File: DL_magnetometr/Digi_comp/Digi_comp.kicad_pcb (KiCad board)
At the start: 2 copper layers, 24 parts, among them J1 Conn_01x06_Male, U1 JST-PHR-2-Connector, U2 HC-06, U3 AP7331-WG-7, U4 ATmega328P-MU

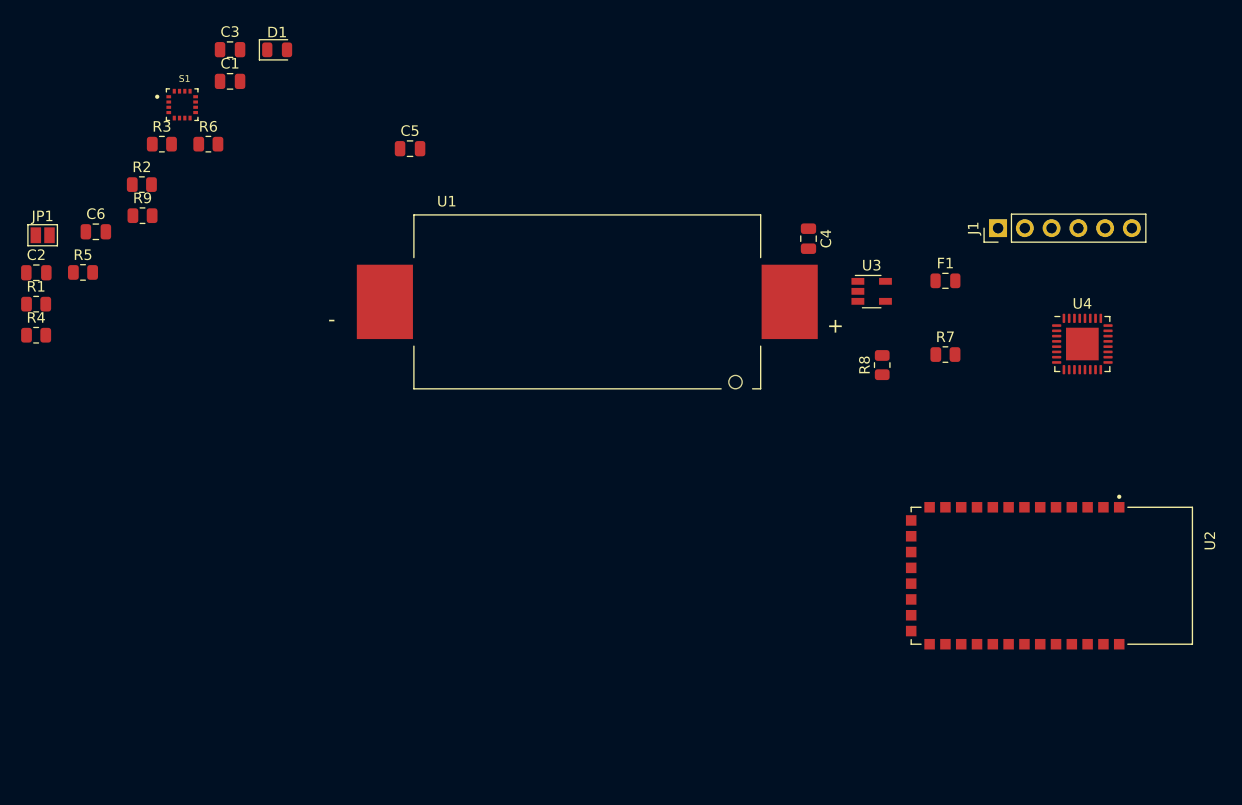
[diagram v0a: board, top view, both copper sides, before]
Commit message: Layout finished
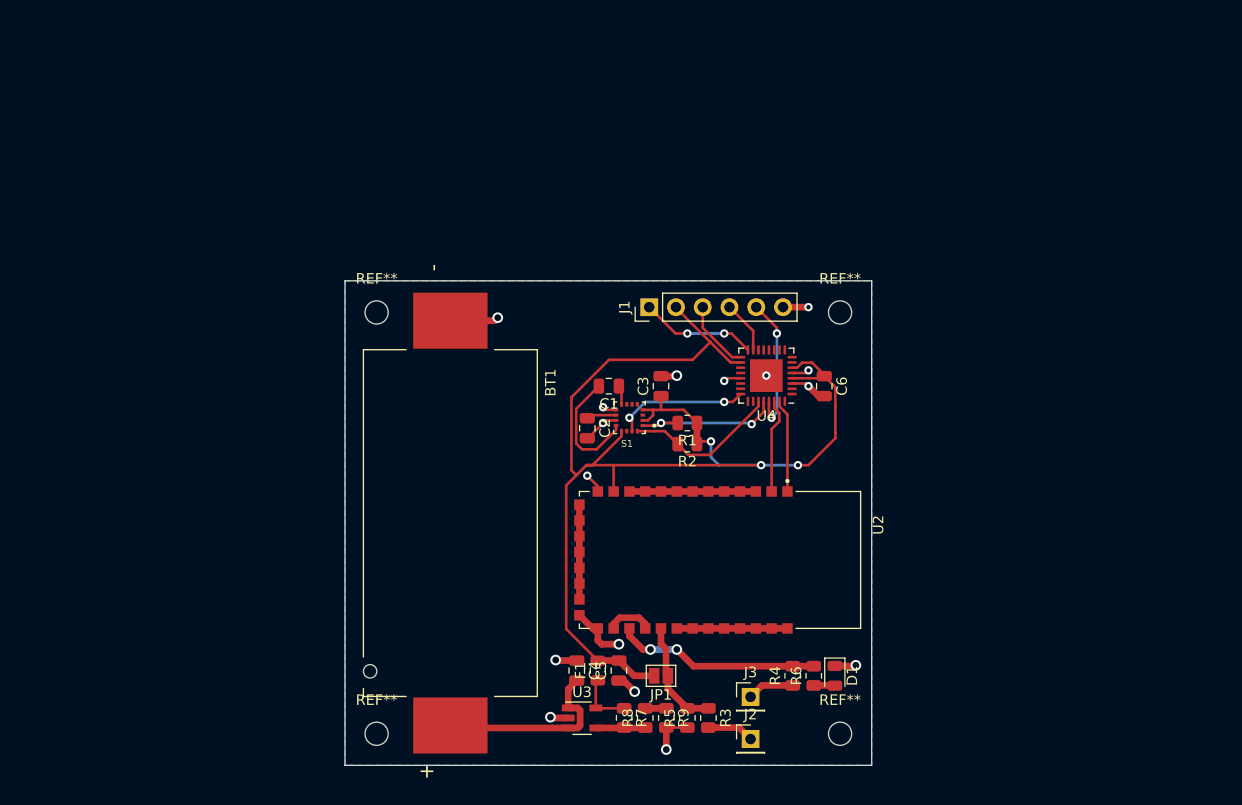
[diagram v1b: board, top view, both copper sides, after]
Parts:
- removed U1: JST-PHR-2-Connector, Dokumenty:2AA-SM
- added BT1: Battery_Cell, Dokumenty:2AA-SM, F.Cu at (75.0, 65.0)
- added J2: Conn_01x01_Male, Connector_PinHeader_2.54mm:PinHeader_1x01_P2.54mm_Vertical, F.Cu at (103.5, 85.5)
- added J3: Conn_01x01_Male, Connector_PinHeader_2.54mm:PinHeader_1x01_P2.54mm_Vertical, F.Cu at (103.5, 81.5)
- added REF**: MountingHole_2.2mm_M2, MountingHole:MountingHole_2.2mm_M2, F.Cu at (112.0, 85.0)
- added REF**: MountingHole_2.2mm_M2, MountingHole:MountingHole_2.2mm_M2, F.Cu at (68.0, 85.0)
- added REF**: MountingHole_2.2mm_M2, MountingHole:MountingHole_2.2mm_M2, F.Cu at (112.0, 45.0)
- added REF**: MountingHole_2.2mm_M2, MountingHole:MountingHole_2.2mm_M2, F.Cu at (68.0, 45.0)
- moved D1 79.6 mm to (111.5, 79.5), turned to 270 degrees
- moved R4 78.8 mm to (107.5, 79.5), turned to 90 degrees
- moved R6 76.5 mm to (109.5, 79.5), turned to 90 degrees
- moved R3 75.2 mm to (99.5, 83.5), turned to 270 degrees
- moved JP1 72.1 mm to (95.0, 79.5), turned to 180 degrees
- moved R5 71.3 mm to (97.5, 83.5), turned to 90 degrees
- moved C6 70.7 mm to (110.5, 52.0), turned to 270 degrees
- moved R9 68.9 mm to (95.5, 83.5), turned to 270 degrees
- moved R1 62.8 mm to (97.5, 55.5), turned to 180 degrees
- moved R2 57.3 mm to (97.5, 57.5), turned to 180 degrees
- moved C2 54.3 mm to (88.0, 56.0), turned to 270 degrees
- moved C5 53.4 mm to (91.0, 79.0), turned to 90 degrees
- moved C3 51.9 mm to (95.0, 52.0), turned to 90 degrees
- moved S1 51.8 mm to (92.0, 55.0), turned to 180 degrees
- moved F1 49.6 mm to (89.0, 79.0), turned to 90 degrees
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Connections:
- R3 pad 2: (no net) -> Net-(J2-Pad1)
- R4 pad 1: (no net) -> Net-(J3-Pad1)
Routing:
- net 3.3V: track 0.00 -> 122.0 mm, vias 0 -> 3
- net GND: track 0.00 -> 39.5 mm, vias 0 -> 16
- net (no net): track 0.00 -> 35.8 mm
- net Net-(R4-Pad2): track 0.00 -> 19.4 mm, vias 0 -> 2
- net 3.6V: track 0.00 -> 18.6 mm
- net SCL: track 0.00 -> 15.1 mm, vias 0 -> 2
- net SDA: track 0.00 -> 14.8 mm
- net Net-(J1-Pad5): track 0.00 -> 13.2 mm, vias 0 -> 2
- net INT: track 0.00 -> 12.9 mm, vias 0 -> 2
- net Net-(C1-Pad2): track 0.00 -> 11.5 mm
- net Net-(J1-Pad1): track 0.00 -> 11.1 mm, vias 0 -> 2
- net Net-(JP1-Pad1): track 0.00 -> 10.8 mm
- net UART_RXD: track 0.00 -> 9.06 mm
- net UART_TXD: track 0.00 -> 8.87 mm
- net Net-(J1-Pad3): track 0.00 -> 6.72 mm
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- added copper zone on B.Cu, net GND
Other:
- board outline added: 50 x 46 mm
- net class Small added: clearance 0.2, trace_width 0.254, via_dia 0.8, via_drill 0.4
